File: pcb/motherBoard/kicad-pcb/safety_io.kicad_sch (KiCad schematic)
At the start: 17 parts, among them J801 ARM KEY, J802 12V VALVE, J803 DEPLOY SWITCH, J804 RECOVERY INPUT, Q801 AO3400A C20917

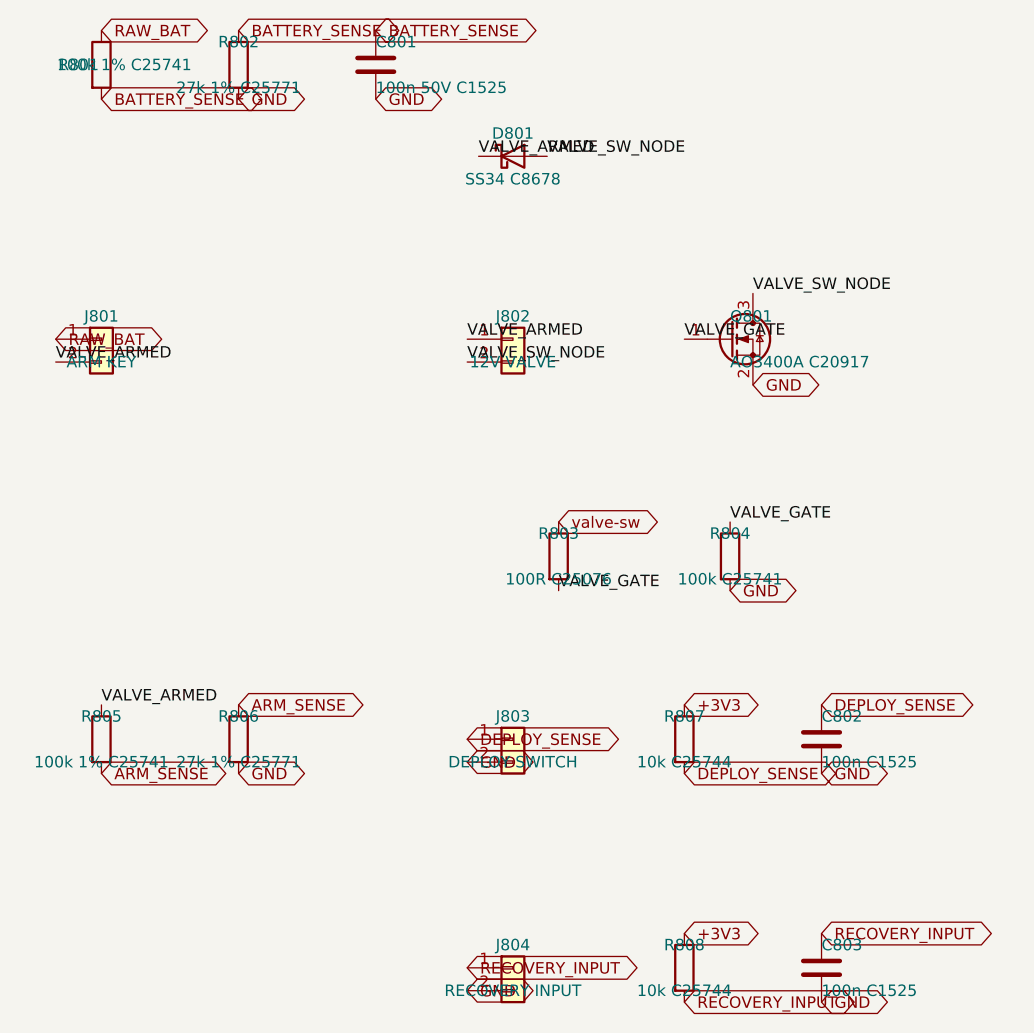
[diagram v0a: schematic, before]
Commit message: chore: little 3d models and code fix
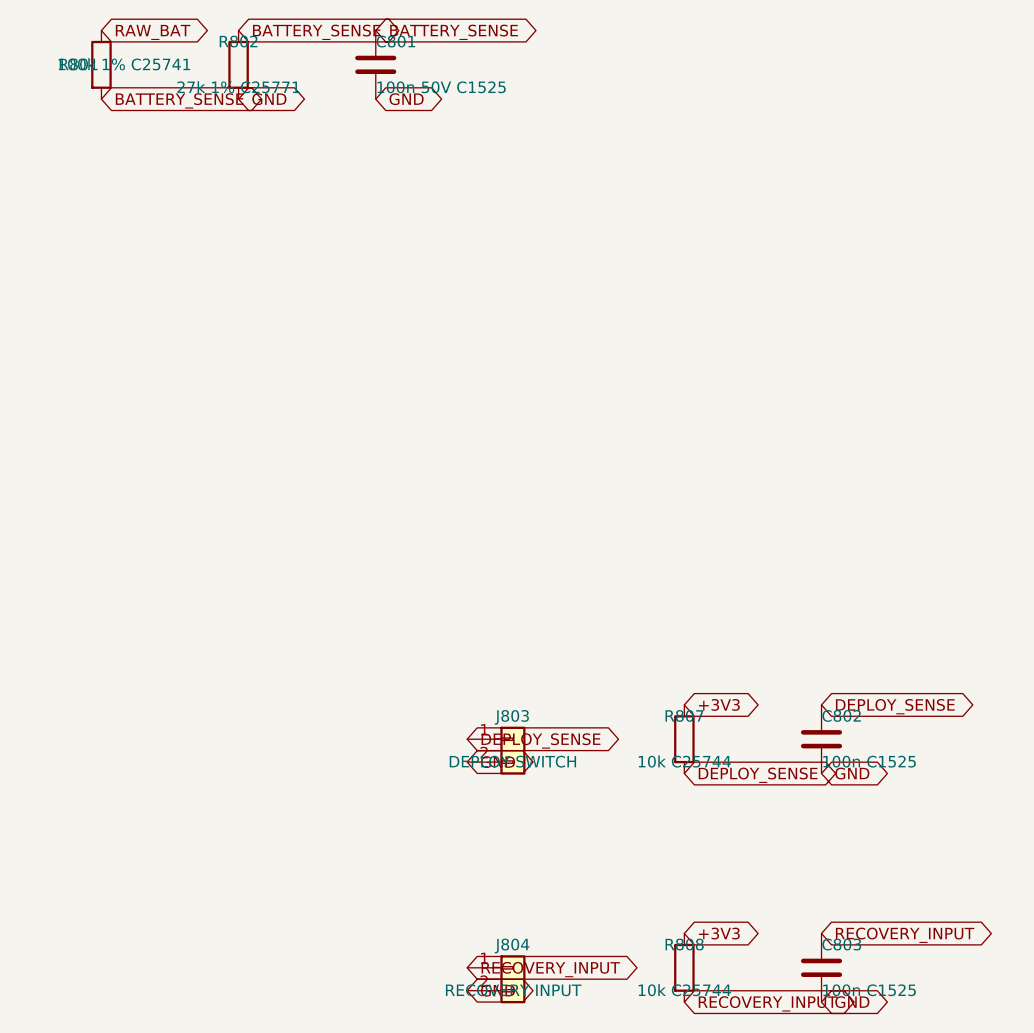
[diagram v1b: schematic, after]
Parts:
- removed D801: SS34 C8678, Diode_SMD:D_SMA, symbol Device:D_Schottky
- removed J801: ARM KEY, TerminalBlock_Altech:Altech_AK100_1x02_P5.00mm, symbol Connector_Generic:Conn_01x02
- removed J802: 12V VALVE, TerminalBlock_Altech:Altech_AK100_1x02_P5.00mm, symbol Connector_Generic:Conn_01x02
- removed Q801: AO3400A C20917, Package_TO_SOT_SMD:SOT-23, symbol Transistor_FET:Q_NMOS_GSD
- removed R803: 100R C25076, Resistor_SMD:R_0402_1005Metric, symbol Device:R
- removed R804: 100k C25741, Resistor_SMD:R_0402_1005Metric, symbol Device:R
- removed R805: 100k 1% C25741, Resistor_SMD:R_0402_1005Metric, symbol Device:R
- removed R806: 27k 1% C25771, Resistor_SMD:R_0402_1005Metric, symbol Device:R
